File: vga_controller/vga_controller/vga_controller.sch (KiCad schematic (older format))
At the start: 0 parts

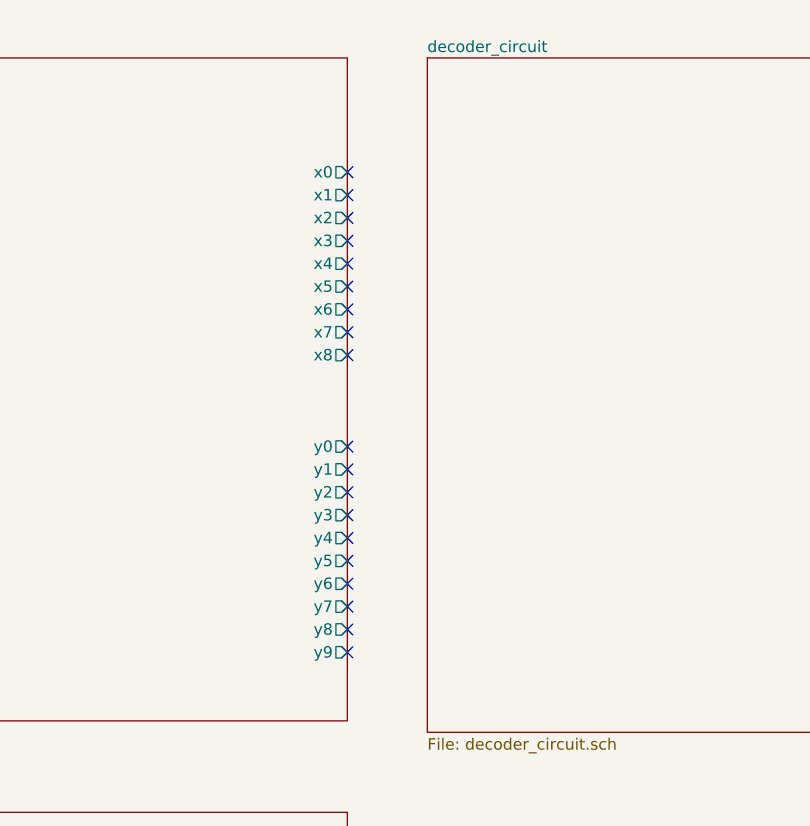
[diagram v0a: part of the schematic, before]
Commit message: made interconnects
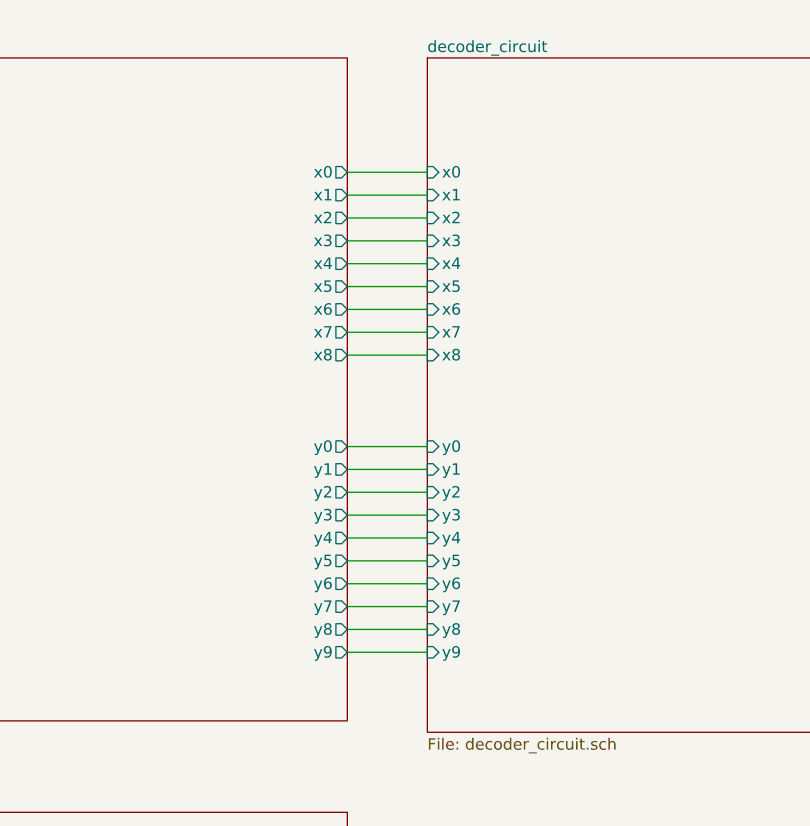
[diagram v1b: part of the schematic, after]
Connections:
- no-connect marks 19 -> 0
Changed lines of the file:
@@
 F0 "decoder_circuit" 50
 F1 "decoder_circuit.sch" 50
+F2 "x0" I L 4650 1200 50
+F3 "x1" I L 4650 1300 50
+F4 "x2" I L 4650 1400 50
+F5 "x3" I L 4650 1500 50
+F6 "x4" I L 4650 1600 50
+F7 "x5" I L 4650 1700 50
+F8 "x6" I L 4650 1800 50
+F9 "x7" I L 4650 1900 50
+F10 "x8" I L 4650 2000 50
+F11 "y0" I L 4650 2400 50
+F12 "y1" I L 4650 2500 50
+F13 "y2" I L 4650 2600 50
+F14 "y3" I L 4650 2700 50
+F15 "y4" I L 4650 2800 50
+F16 "y5" I L 4650 2900 50
+F17 "y6" I L 4650 3000 50
+F18 "y7" I L 4650 3100 50
+F19 "y8" I L 4650 3200 50
+F20 "y9" I L 4650 3300 50
 $EndSheet
 $Sheet
@@
 F1 "pixel_memory.sch" 50
 $EndSheet
+$Comp
+L power:+5V #PWR01
+U 1 1 5E772D7F
+P 10250 750
+F 0 "#PWR01" H 10250 600 50  0001 C CNN
+F 1 "+5V" H 10265 923 50  0000 C CNN
+F 2 "" H 10250 750 50  0001 C CNN
+F 3 "" H 10250 750 50  0001 C CNN
+	1    10250 750
+	1    0    0    -1
+$EndComp
+$Comp
+L power:GND #PWR02
+U 1 1 5E77329E
+P 10250 1200
+F 0 "#PWR02" H 10250 950 50  0001 C CNN
+F 1 "GND" H 10255 1027 50  0000 C CNN
+F 2 "" H 10250 1200 50  0001 C CNN
+F 3 "" H 10250 1200 50  0001 C CNN
+	1    10250 1200
+	1    0    0    -1
+$EndComp
+$Comp
+L power:PWR_FLAG #FLG01
+U 1 1 5E77346B
+P 10250 750
+F 0 "#FLG01" H 10250 825 50  0001 C CNN
+F 1 "PWR_FLAG" H 10250 923 50  0000 C CNN
+F 2 "" H 10250 750 50  0001 C CNN
+F 3 "~" H 10250 750 50  0001 C CNN
+	1    10250 750
+	-1   0    0    1
+$EndComp
+$Comp
+L power:PWR_FLAG #FLG02
+U 1 1 5E773925
+P 10250 1200
+F 0 "#FLG02" H 10250 1275 50  0001 C CNN
+F 1 "PWR_FLAG" H 10250 1373 50  0000 C CNN
+F 2 "" H 10250 1200 50  0001 C CNN
+F 3 "~" H 10250 1200 50  0001 C CNN
+	1    10250 1200
+	1    0    0    -1
+$EndComp
+Wire Wire Line
+	4300 1200 4650 1200
+Wire Wire Line
+	4300 1300 4650 1300
+Wire Wire Line
+	4300 1400 4650 1400
+Wire Wire Line
+	4300 1500 4650 1500
+Wire Wire Line
+	4300 1600 4650 1600
+Wire Wire Line
+	4300 1700 4650 1700
+Wire Wire Line
+	4300 1800 4650 1800
+Wire Wire Line
+	4300 1900 4650 1900
+Wire Wire Line
+	4300 2000 4650 2000
 $Sheet
 S 800  700  3500 2900
@@
 F20 "x0" O R 4300 1200 50
 $EndSheet
-NoConn ~ 4300 1200
-NoConn ~ 4300 1300
-NoConn ~ 4300 1400
-NoConn ~ 4300 1500
-NoConn ~ 4300 1600
-NoConn ~ 4300 1700
-NoConn ~ 4300 1800
-NoConn ~ 4300 1900
-NoConn ~ 4300 2000
-NoConn ~ 4300 2400
-NoConn ~ 4300 2500
-NoConn ~ 4300 2600
-NoConn ~ 4300 2700
-NoConn ~ 4300 2800
-NoConn ~ 4300 2900
-NoConn ~ 4300 3000
-NoConn ~ 4300 3100
-NoConn ~ 4300 3200
-NoConn ~ 4300 3300
-$Comp
-L power:+5V #PWR0105
-U 1 1 5E772D7F
-P 10250 750
-F 0 "#PWR0105" H 10250 600 50  0001 C CNN
-F 1 "+5V" H 10265 923 50  0000 C CNN
-F 2 "" H 10250 750 50  0001 C CNN
-F 3 "" H 10250 750 50  0001 C CNN
-	1    10250 750
-	1    0    0    -1
-$EndComp
-$Comp
-L power:GND #PWR0106
-U 1 1 5E77329E
-P 10250 1200
-F 0 "#PWR0106" H 10250 950 50  0001 C CNN
-F 1 "GND" H 10255 1027 50  0000 C CNN
-F 2 "" H 10250 1200 50  0001 C CNN
-F 3 "" H 10250 1200 50  0001 C CNN
-	1    10250 1200
-	1    0    0    -1
-$EndComp
-$Comp
-L power:PWR_FLAG #FLG0101
-U 1 1 5E77346B
-P 10250 750
-F 0 "#FLG0101" H 10250 825 50  0001 C CNN
-F 1 "PWR_FLAG" H 10250 923 50  0000 C CNN
-F 2 "" H 10250 750 50  0001 C CNN
-F 3 "~" H 10250 750 50  0001 C CNN
-	1    10250 750
-	-1   0    0    1
-$EndComp
-$Comp
-L power:PWR_FLAG #FLG0102
-U 1 1 5E773925
-P 10250 1200
-F 0 "#FLG0102" H 10250 1275 50  0001 C CNN
-F 1 "PWR_FLAG" H 10250 1373 50  0000 C CNN
-F 2 "" H 10250 1200 50  0001 C CNN
-F 3 "~" H 10250 1200 50  0001 C CNN
-	1    10250 1200
-	1    0    0    -1
-$EndComp
+Wire Wire Line
+	4300 2400 4650 2400
+Wire Wire Line
+	4300 2500 4650 2500
+Wire Wire Line
+	4300 2600 4650 2600
+Wire Wire Line
+	4300 2700 4650 2700
+Wire Wire Line
+	4300 2800 4650 2800
+Wire Wire Line
+	4300 2900 4650 2900
+Wire Wire Line
+	4300 3000 4650 3000
+Wire Wire Line
+	4300 3100 4650 3100
+Wire Wire Line
+	4300 3200 4650 3200
+Wire Wire Line
+	4300 3300 4650 3300
 $EndSCHEMATC
